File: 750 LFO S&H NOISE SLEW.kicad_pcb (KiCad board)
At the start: 2 copper layers, 65 x 106.5 mm, 242 parts, among them J1 PJ301BM, J10 PJ301BM, J11 PJ301BM, J2 PJ301BM, J3 PJ301BM, J4 PJ301BM, J5 JACK_MONO_SW, J6 PJ301BM, J7 JACK_MONO_SW, J8 PJ301BM, J9 PJ301BM, P1 CONN_01X03, P3 CONN_02X05, Q1 MMBT3904, Q10 MMBT3904, Q11 J112, Q12 MMBT3906, Q13 J112, Q14 J112, Q15 MMBT3904, Q16 MMBT3904, Q2 MMBT3904, Q3 2N7002, Q4 2N7002, Q5 MBT3946DW, Q6 MBT3946DW, Q7 MMBT3904, Q8 MMBT3904, Q9 MMBT3904, SW1 KS-01Q, SW2 KS-01Q, SW3 SPDT, U1 LM13700, U10 TL072-, U11 TL072-, U12 MAX9945, U13 DG409, U14 DG409, U15 TS321, U2 TL072-, U3 TL072-, U4 TL072-, U5 TL072-, U6 CD40106, U7 CD4027, U8 CD4027, U9 TL072-

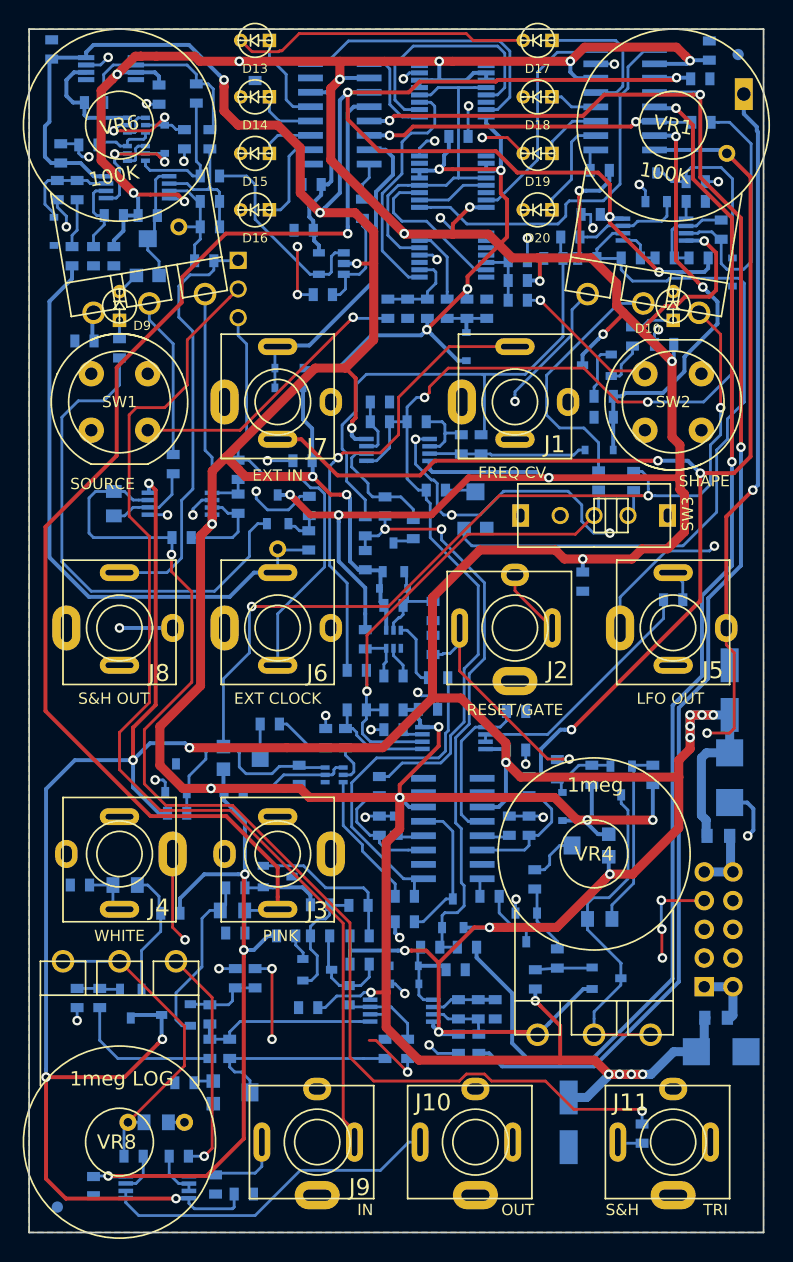
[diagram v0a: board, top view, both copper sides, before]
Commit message: tweakings
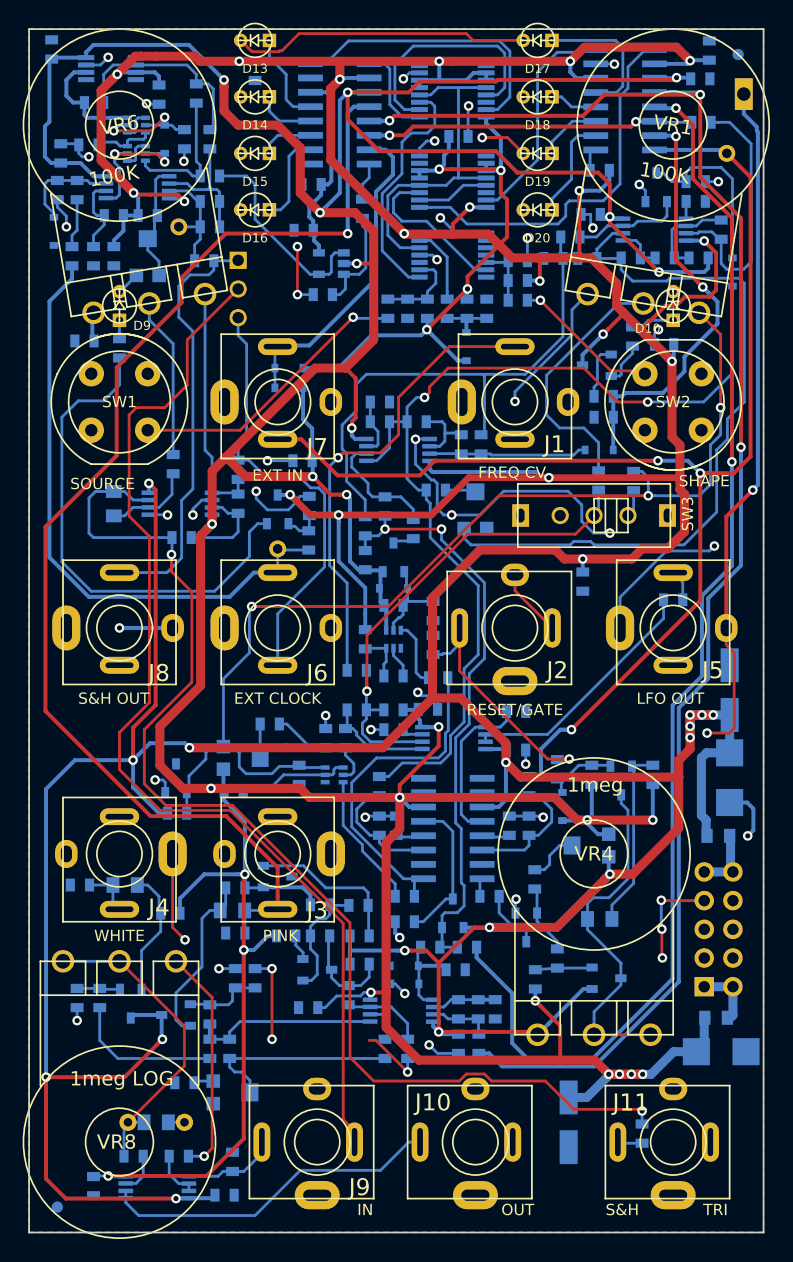
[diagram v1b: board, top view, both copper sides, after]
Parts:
- moved R100 2.50 mm to (78.0, 125.2), turned to 90 degrees
- moved C19 1.70 mm to (77.3, 128.2)
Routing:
- net +12V: track 651.0 -> 647.6 mm
- net Net-(J9-Pad3): track 9.05 -> 8.29 mm
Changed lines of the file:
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@@
     (links 506)
     (no_connects 0)
-    (area 59.924999 24.924999 125.075001 131.575001)
+    (area 56.936905 22.45604 128.313095 132.325001)
     (thickness 1.6)
     (drawings 943)
-    (tracks 2020)
+    (tracks 2019)
     (zones 0)
     (modules 242)
@@
   )
   (module MyModules:SM0603-C-JRL (layer B.Cu)
-    (at 79 128.1)
+    (at 77.3 128.2)
     (attr smd)
     (fp_text reference C19 (at 2 0 90) (layer B.SilkS)
@@
   )
   (module MyModules:SM0603-R-JRL (layer B.Cu)
-    (at 76.5 127.25 270)
+    (at 78 125.25 90)
     (attr smd)
-    (fp_text reference R100 (at -1.85 -0.5 360) (layer B.SilkS)
+    (fp_text reference R100 (at 0 1.4 270) (layer B.SilkS)
       (effects (font (size 0.6096 0.6096) (thickness 0.1524)) (justify mirror))
     )
-    (fp_text value 1meg (at 0 0 270) (layer B.SilkS) hide
+    (fp_text value 1meg (at 0 0 90) (layer B.SilkS) hide
       (effects (font (size 0.508 0.4572) (thickness 0.1143)) (justify mirror))
     )
@@
     (fp_line (start 0.5 0.8) (end 1.4 0.8) (layer B.SilkS) (width 0.2))
     (fp_line (start 0.5 -0.8) (end 1.4 -0.8) (layer B.SilkS) (width 0.2))
-    (pad 1 smd rect (at -0.8509 0 270) (size 0.8128 1.143) (layers B.Cu B.Paste B.Mask)
+    (pad 1 smd rect (at -0.8509 0 90) (size 0.8128 1.143) (layers B.Cu B.Paste B.Mask)
       (net 62 "Net-(J9-Pad3)"))
-    (pad 2 smd rect (at 0.8509 0 270) (size 0.8128 1.143) (layers B.Cu B.Paste B.Mask)
+    (pad 2 smd rect (at 0.8509 0 90) (size 0.8128 1.143) (layers B.Cu B.Paste B.Mask)
       (net 1 GND))
     (model Resistors_SMD.3dshapes/R_0603.wrl
@@
     (at 73.25 124.75 180)
     (attr smd)
-    (fp_text reference R104 (at -3.05 0.85 180) (layer B.SilkS)
+    (fp_text reference R104 (at -2.75 0.95 180) (layer B.SilkS)
       (effects (font (size 0.6096 0.6096) (thickness 0.1524)) (justify mirror))
     )
@@
   (module MyModules:CAP-5MM-BOX-0805-COMBO (layer B.Cu)
     (at 71.25 121.75)
-    (fp_text reference C44 (at 4.4 0 90) (layer B.SilkS)
+    (fp_text reference C44 (at -4.45 -0.05 270) (layer B.SilkS)
       (effects (font (size 0.8128 0.8128) (thickness 0.1524)) (justify mirror))
     )
@@
   (segment (start 90.05 105.1991) (end 90.05 102.5991) (width 0.25) (layer B.Cu) (net 3))
   (segment (start 90.05 102.5991) (end 90.0009 102.55) (width 0.25) (layer B.Cu) (net 3))
+  (segment (start 74.144 128.4681) (end 76.181 128.4681) (width 0.35) (layer B.Cu) (net 4))
+  (segment (start 76.181 128.4681) (end 76.4491 128.2) (width 0.35) (layer B.Cu) (net 4))
   (segment (start 69.2 89.699998) (end 70.699998 88.2) (width 0.35) (layer B.Cu) (net 4))
   (segment (start 70.699998 88.2) (end 73.8 88.2) (width 0.35) (layer B.Cu) (net 4))
@@
   (segment (start 78.6018 27.8491) (end 78.6 27.8509) (width 0.35) (layer B.Cu) (net 4))
   (via (at 78.6 27.8509) (size 0.85) (drill 0.45) (layers F.Cu B.Cu) (net 4))
-  (segment (start 78 129.4) (end 78.1491 129.2509) (width 0.25) (layer B.Cu) (net 4))
-  (segment (start 78.1491 129.2509) (end 78.1491 128.1) (width 0.25) (layer B.Cu) (net 4))
-  (segment (start 74.6259 129.4) (end 78 129.4) (width 0.25) (layer B.Cu) (net 4))
-  (segment (start 74.144 128.4681) (end 74.144 128.9181) (width 0.25) (layer B.Cu) (net 4))
-  (segment (start 74.144 128.9181) (end 74.6259 129.4) (width 0.25) (layer B.Cu) (net 4))
   (segment (start 98 113.9491) (end 96.4491 113.9491) (width 0.35) (layer B.Cu) (net 4))
   (segment (start 96.4491 113.9491) (end 96.25 113.75) (width 0.35) (layer B.Cu) (net 4))
@@
   (segment (start 76.3509 45.5) (end 78.46 45.5) (width 0.25) (layer B.Cu) (net 60))
   (segment (start 78.46 45.5) (end 78.5 45.46) (width 0.25) (layer B.Cu) (net 60))
-  (segment (start 76.5 126.3991) (end 76.6491 126.3991) (width 0.25) (layer B.Cu) (net 62))
-  (segment (start 76.75 126.5) (end 77 126.25) (width 0.25) (layer B.Cu) (net 62))
-  (segment (start 76.6491 126.3991) (end 76.75 126.5) (width 0.25) (layer B.Cu) (net 62))
-  (segment (start 77 126.25) (end 80 126.25) (width 0.25) (layer B.Cu) (net 62))
-  (segment (start 80 126.25) (end 80.6 125.65) (width 0.25) (layer B.Cu) (net 62))
-  (segment (start 80.6 125.65) (end 80.6 123.5) (width 0.25) (layer B.Cu) (net 62))
-  (segment (start 74.144 126.525) (end 76.3741 126.525) (width 0.25) (layer B.Cu) (net 62))
-  (segment (start 76.3741 126.525) (end 76.5 126.3991) (width 0.25) (layer B.Cu) (net 62))
+  (segment (start 78 126.1009) (end 78.9991 126.1009) (width 0.25) (layer B.Cu) (net 62))
+  (segment (start 78.9991 126.1009) (end 80.6 124.5) (width 0.25) (layer B.Cu) (net 62))
+  (segment (start 80.6 124.5) (end 80.6 123.5) (width 0.25) (layer B.Cu) (net 62))
+  (segment (start 76.725 126.525) (end 77.1491 126.1009) (width 0.25) (layer B.Cu) (net 62))
+  (segment (start 77.1491 126.1009) (end 78 126.1009) (width 0.25) (layer B.Cu) (net 62))
+  (segment (start 74.144 126.525) (end 76.725 126.525) (width 0.25) (layer B.Cu) (net 62))
   (segment (start 68.556 128.4554) (end 68.556 128.85526) (width 0.25) (layer B.Cu) (net 63))
   (segment (start 68.556 128.85526) (end 69.70074 130) (width 0.25) (layer B.Cu) (net 63))
@@
   (segment (start 98.865 95.115) (end 100.09842 95.115) (width 0.25) (layer B.Cu) (net 106))
   (segment (start 98.5 69.2) (end 98.5 70.05) (width 0.25) (layer B.Cu) (net 107))
-  (segment (start 98.5 70.05) (end 99.181401 70.731401) (width 0.25) (layer B.Cu) (net 107))
-  (segment (start 99.181401 70.731401) (end 117.868599 70.731401) (width 0.25) (layer B.Cu) (net 107))
-  (segment (start 116.699989 47.050011) (end 116.449999 47.300001) (width 0.25) (layer B.Cu) (net 107))
-  (segment (start 117.868599 70.731401) (end 120.849997 67.750003) (width 0.25) (layer B.Cu) (net 107))
-  (segment (start 120.849997 67.750003) (end 120.849997 62.250003) (width 0.25) (layer B.Cu) (net 107))
+  (segment (start 121.8 59.5) (end 123.3 58) (width 0.25) (layer B.Cu) (net 107))
+  (segment (start 98.5 70.05) (end 99.1 70.65) (width 0.25) (layer B.Cu) (net 107))
+  (segment (start 99.1 70.65) (end 107.9 70.65) (width 0.25) (layer B.Cu) (net 107))
+  (segment (start 110 70.65) (end 117.95 70.65) (width 0.25) (layer B.Cu) (net 107))
+  (segment (start 107.9 70.65) (end 108.2 70.35) (width 0.25) (layer B.Cu) (net 107))
+  (segment (start 121.8 61.3) (end 121.8 59.5) (width 0.25) (layer B.Cu) (net 107))
+  (segment (start 109.7 70.35) (end 110 70.65) (width 0.25) (layer B.Cu) (net 107))
   (segment (start 123.3 58) (end 123.3 47.5) (width 0.25) (layer B.Cu) (net 107))
-  (segment (start 120.849997 62.250003) (end 121.8 61.3) (width 0.25) (layer B.Cu) (net 107))
+  (segment (start 108.2 70.35) (end 109.7 70.35) (width 0.25) (layer B.Cu) (net 107))
   (segment (start 113.400001 47.300001) (end 112.3991 46.2991) (width 0.25) (layer B.Cu) (net 107))
-  (segment (start 121.8 61.3) (end 121.8 59.5) (width 0.25) (layer B.Cu) (net 107))
-  (segment (start 121.8 59.5) (end 123.3 58) (width 0.25) (layer B.Cu) (net 107))
+  (segment (start 117.95 70.65) (end 120.849997 67.750003) (width 0.25) (layer B.Cu) (net 107))
+  (segment (start 120.849997 67.750003) (end 120.849997 62.250003) (width 0.25) (layer B.Cu) (net 107))
+  (segment (start 116.699989 47.050011) (end 116.449999 47.300001) (width 0.25) (layer B.Cu) (net 107))
+  (segment (start 120.849997 62.250003) (end 121.8 61.3) (width 0.25) (layer B.Cu) (net 107))
   (segment (start 123.3 47.5) (end 122.850011 47.050011) (width 0.25) (layer B.Cu) (net 107))
   (segment (start 122.850011 47.050011) (end 116.699989 47.050011) (width 0.25) (layer B.Cu) (net 107))
